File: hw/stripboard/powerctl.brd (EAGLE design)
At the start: 43.2 x 62.2 mm, 15 parts, among them J3 JST-B3B-XH, U1 ATTiny85P

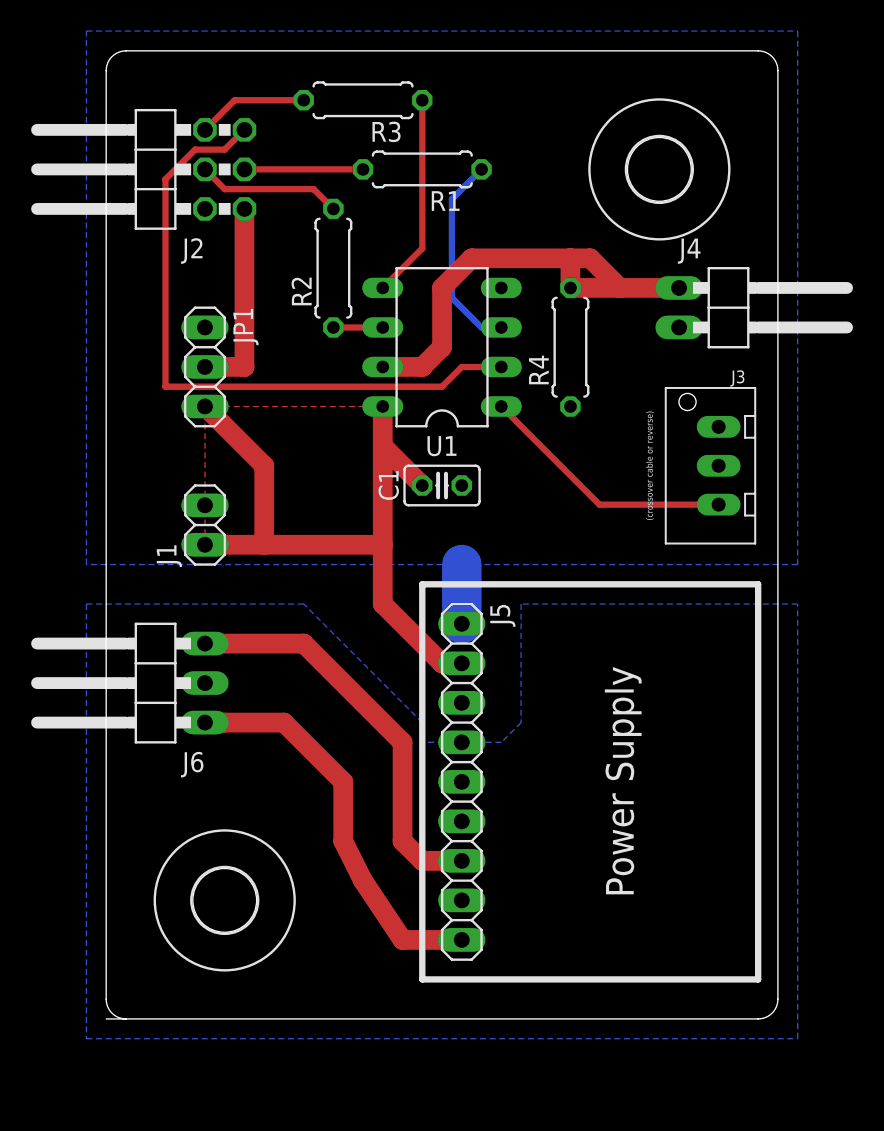
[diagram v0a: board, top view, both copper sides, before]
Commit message: hw: add PCB hardware definition and CAM files
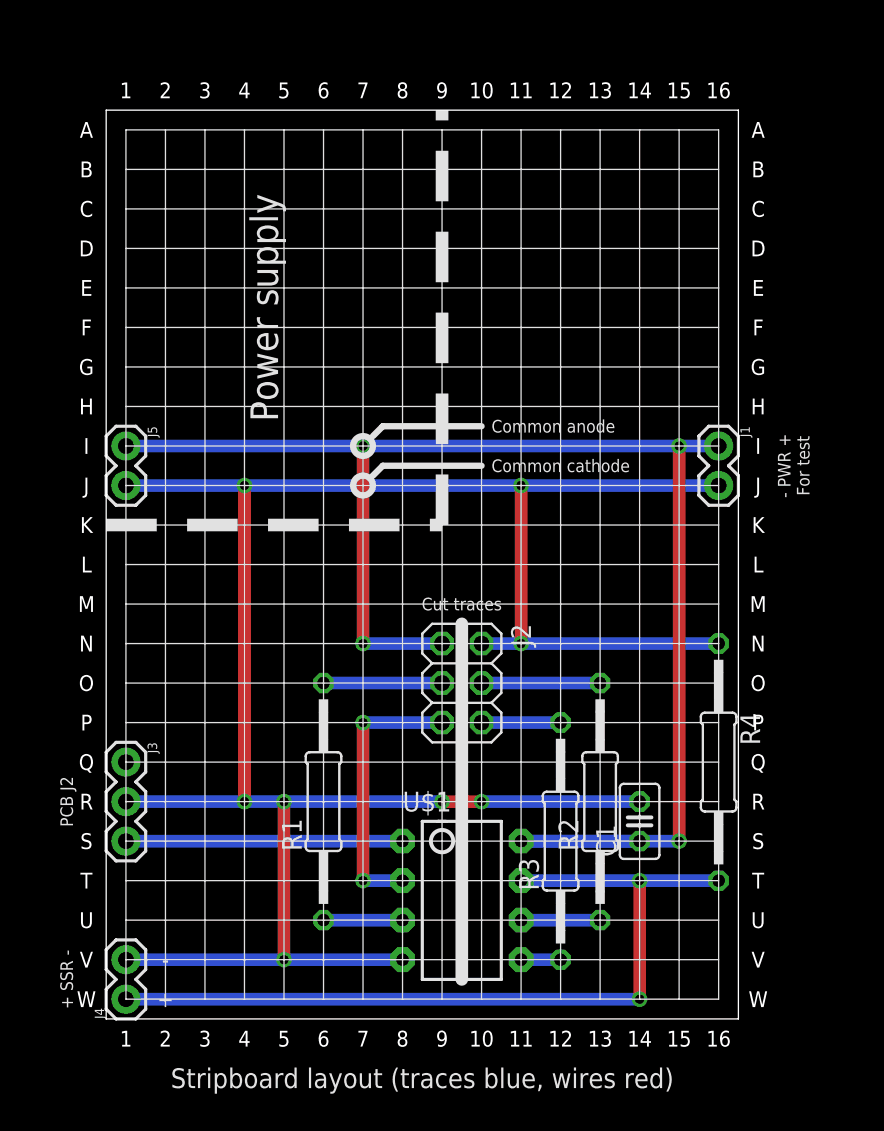
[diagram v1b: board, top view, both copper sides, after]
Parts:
- removed H1, H2: MOUNT-HOLE4.1, holes:4,1
- removed J6: (no value), pinhead:1X03/90
- removed JP1: (no value), pinhead:1X03
- removed U1: ATTiny85P, SparkFun:DIL8
- added U$1: ATTINY85-PU, SparkFun:DIP08
- J1: device pinhead:1X02 -> SparkFun-Connectors:1X02
- J2: value (none) -> MA03-2; device pinhead:2X03/90 -> pinhead:2X03
- J3: value JST-B3B-XH -> JST-XT-3P; device jst-xh:JST-XH-3V -> SparkFun-Connectors:1X03
- J4: device pinhead:1X02/90 -> SparkFun-Connectors:1X02
- J5: device pinhead:1X09 -> SparkFun-Connectors:1X02
- R1, R2, R3, R4: device rcl:0207/7 -> rcl:0207/15
- moved J4 59.4 mm to (1.27, 1.27), turned to 90 degrees
- moved R3 49.3 mm to (29.2, 11.4), turned to 90 degrees
- moved J3 42.6 mm to (1.27, 16.5), turned to 270 degrees
- moved R1 41.1 mm to (14.0, 14.0), turned to 90 degrees
- moved J2 38.8 mm to (22.9, 21.6), turned to 270 degrees
- moved R2 38.3 mm to (31.8, 14.0)
- moved J1 33.4 mm to (39.4, 36.8), turned to 270 degrees
- moved J5 30.5 mm to (1.27, 36.8)
- moved R4 28.3 mm to (39.4, 16.5), turned to 270 degrees
- moved C1 25.0 mm to (34.3, 12.7), turned to 90 degrees
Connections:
- net LEDBO renamed N$1
- net LEDGO renamed N$3
- net LEDRO renamed N$2
- removed net AC-L: J5.9, J6.1
- removed net AC-N: J5.7, J6.3
- removed net LEDCO: J2.1, JP1.2
- removed net PE: J5.4, J5.5, J5.6, J5.8, J6.2
- net !OFF: now also U$1.1; no longer U1.1
- net +5V: now also J2.1, J5.1, U$1.8; no longer J5.2, JP1.3, U1.8
- net BUTTON: now also U$1.2; no longer U1.2
- net GND: now also J5.2, U$1.4; no longer J5.1, JP1.1, U1.4
- net LEDB: now also U$1.5; no longer U1.5
- net LEDG: now also U$1.6; no longer U1.6
- net LEDR: now also U$1.3; no longer U1.3
- net SSR: now also U$1.7; no longer U1.7
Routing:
- net GND: track 3.81 -> 144.8 mm, vias 0 -> 8
- net +5V: track 53.7 -> 99.1 mm, vias 0 -> 4
- net AC-L: track 26.8 -> 0.00 mm
- net AC-N: track 26.0 -> 0.00 mm
- net BUTTON: track 41.8 -> 17.8 mm, vias 0 -> 2
- net SSR: track 30.0 -> 53.3 mm, vias 0 -> 2
- net LEDCO: track 12.7 -> 0.00 mm
- net LEDB: track 13.1 -> 2.54 mm
- net LEDR: track 13.0 -> 5.08 mm
- net N$1: track 7.14 -> 5.08 mm
- net LEDG: track 3.18 -> 5.08 mm
- net N$3: track 9.31 -> 7.62 mm
- net !OFF: track 16.6 -> 17.8 mm
- removed copper zone on layer 1, net +5V
- removed copper zone on layer 16, net GND
- removed copper zone on layer 16, net PE
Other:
- board size 43.2 x 62.2 mm -> 40.6 x 58.4 mm
- board text added: "+ SSR -"
- board text added: "- PWR + For test"
- board text added: "1"
- board text added: "10"
- board text added: "11"
- board text added: "12"
- board text added: "13"
- board text added: "14"
- board text added: "15"
- board text added: "16"
- board text added: "2"
- board text added: "3"
- board text added: "4"
- board text added: "5"
- board text added: "6"
- board text added: "7"
- board text added: "8"
- board text added: "9"
- board text added: "A"
- board text added: "C"
- board text added: "Common anode"
- board text added: "Common cathode"
- board text added: "Cut traces"
- board text added: "D"
- board text added: "E"
- board text added: "F"
- board text added: "H"
- board text added: "I"
- board text added: "J"
- board text added: "K"
- board text added: "M"
- board text added: "O"
- board text added: "P"
- board text added: "PCB J2"
- board text added: "Power supply"
- board text added: "Q"
- board text added: "S"
- board text added: "Stripboard layout (traces blue, wires red)"
- board text added: "T"
- board text added: "U"
- board text added: "V"
- board text added: "W"
- board text removed: "(crossover cable or reverse)"
- board text removed: "5V"
- board text removed: "AC N L"
- board text removed: "BTN"
- board text removed: "BTN GND"
- board text removed: "CA"
- board text removed: "CC"
- board text removed: "J3"
- board text removed: "JST-B3B-XH"
- board text removed: "LED COM"
- board text removed: "LED polarity"
- board text removed: "Mainboard"
- board text removed: "PE"
- board text removed: "Power Supply"
- board text removed: "SSR"
- board text removed: "SSR Pushbutton Controller v 1.0 (C) 2024 H. Peter Anvin"
